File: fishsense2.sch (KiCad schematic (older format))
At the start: 15 parts, among them J1 Conn_02x10_Odd_Even, J10 USB_B_Micro, J5 USB3_A, J6 USB3_A, J7 USB3_A, J8 USB3_A, J9 Barrel_Jack, Q1 Q_NMOS_GSD, SW1 SW_Reed

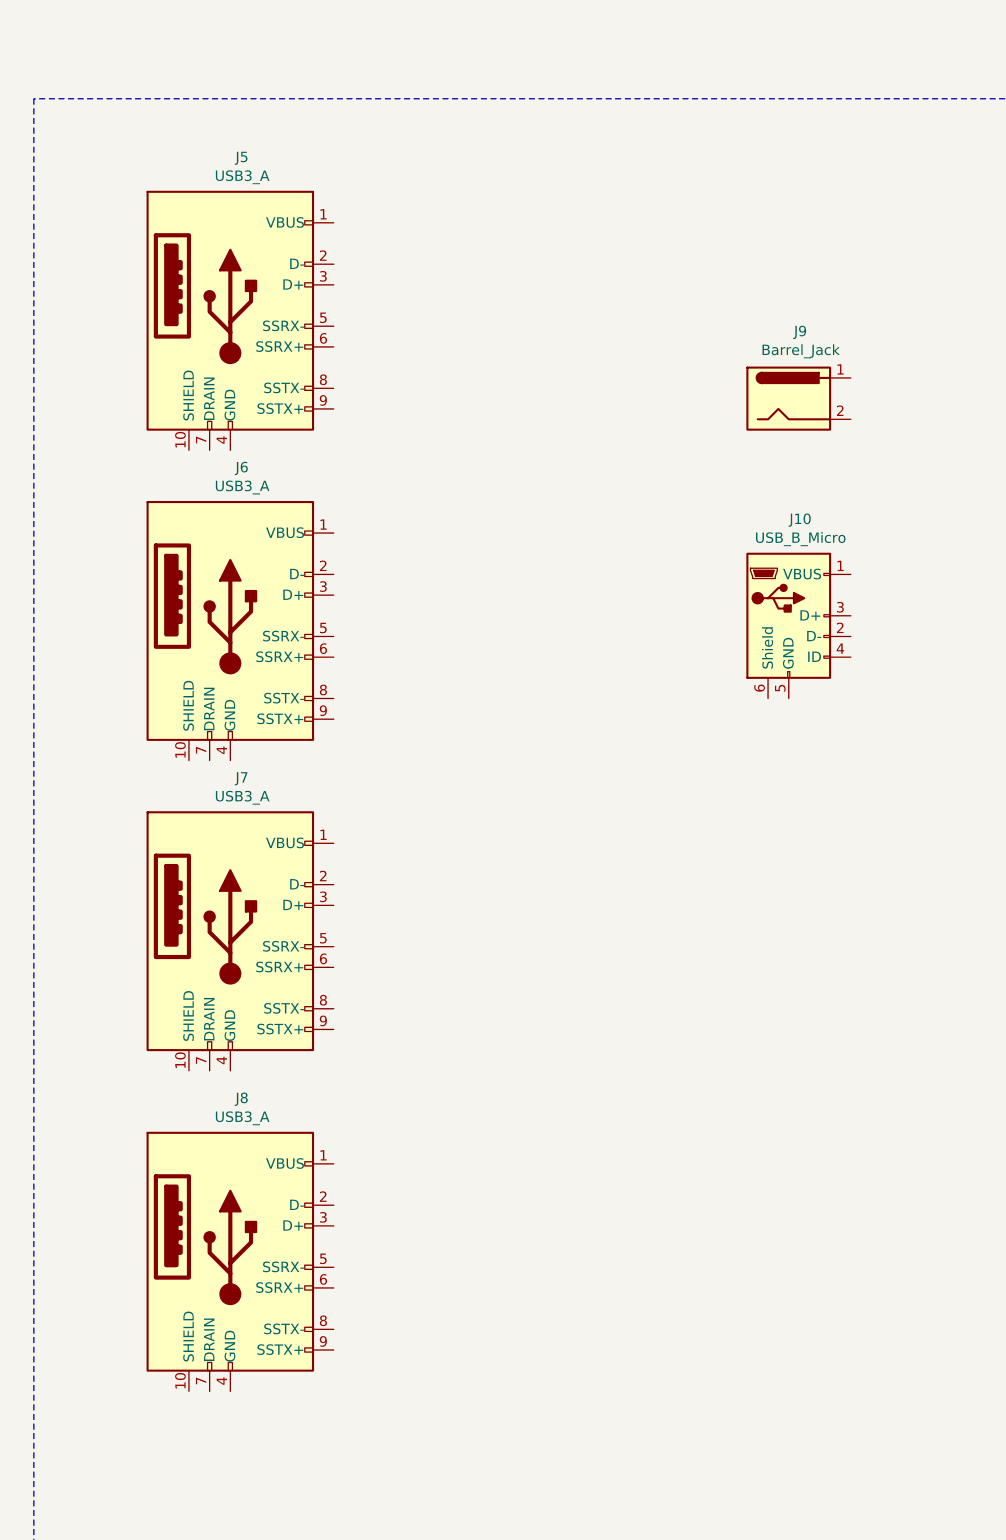
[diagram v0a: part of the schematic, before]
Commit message: Routed traces.
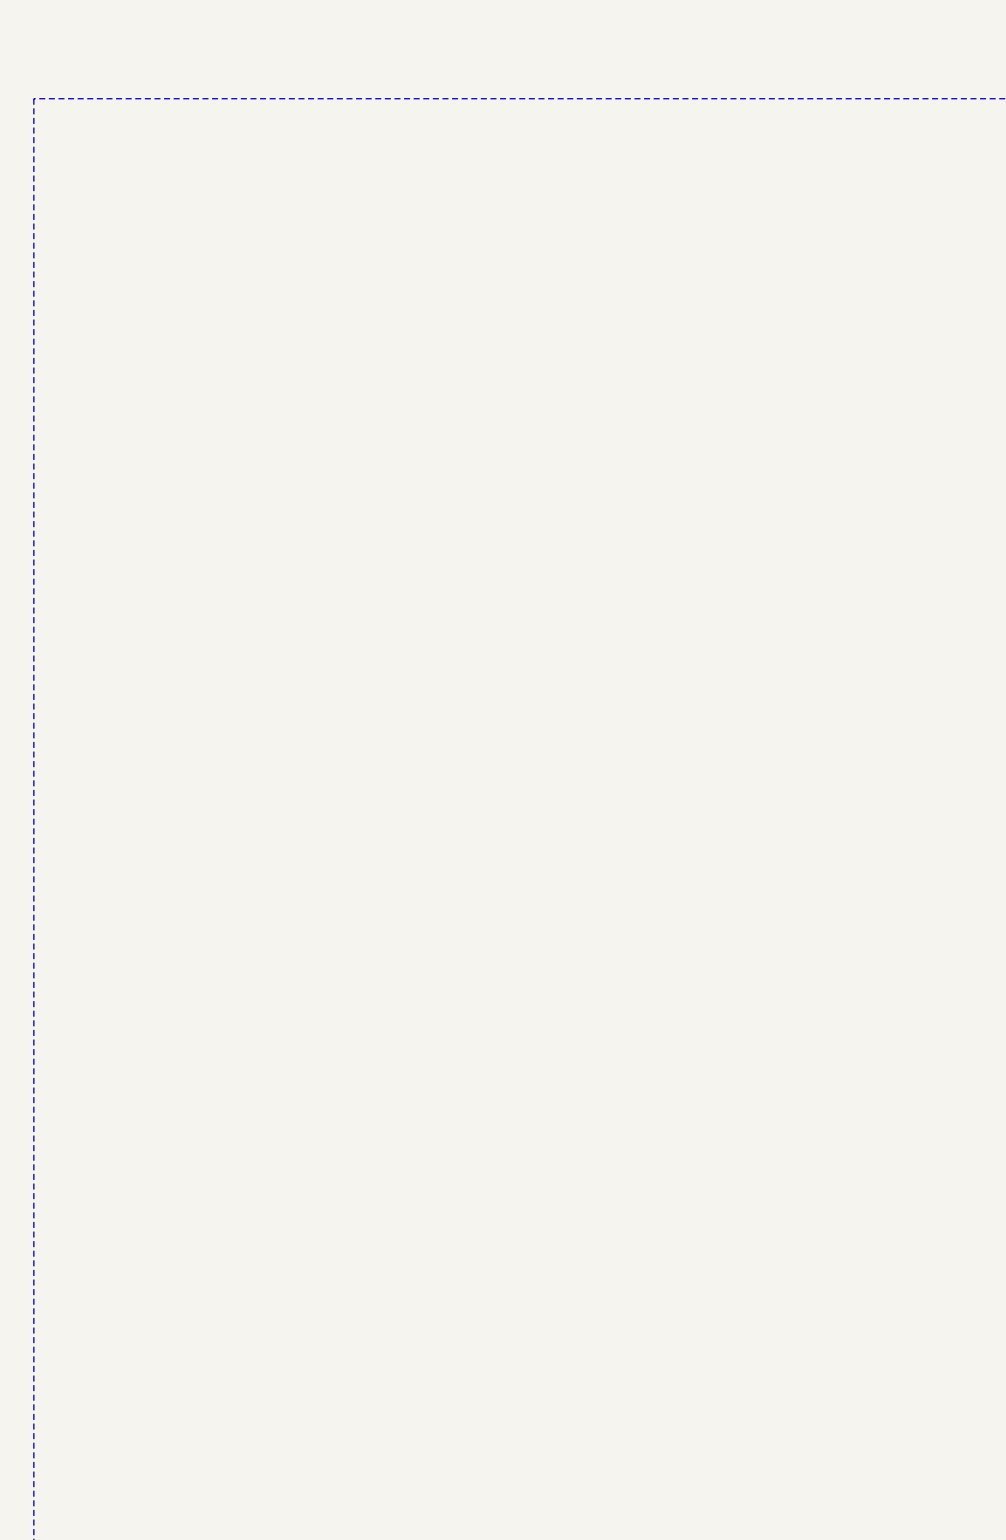
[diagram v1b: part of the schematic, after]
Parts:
- removed J10: USB_B_Micro, Connector_USB:USB_Micro-B_GCT_USB3076-30-A, symbol Connector:USB_B_Micro
- removed J5, J6, J7, J8: USB3_A, Connector_USB:USB3_A_Molex_48393-001, symbol Connector:USB3_A
- removed J9: Barrel_Jack, Connector_BarrelJack:BarrelJack_Horizontal, symbol Connector:Barrel_Jack
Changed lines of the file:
@@
 	11250 1900 4650 1900
-$Comp
-L Connector:USB3_A J5
-U 1 1 6196CE86
-P 5600 2900
-F 0 "J5" H 5657 3617 50  0000 C CNN
-F 1 "USB3_A" H 5657 3526 50  0000 C CNN
-F 2 "Connector_USB:USB3_A_Molex_48393-001" H 5750 3000 50  0001 C CNN
-F 3 "~" H 5750 3000 50  0001 C CNN
-	1    5600 2900
-	1    0    0    -1
-$EndComp
-$Comp
-L Connector:USB3_A J6
-U 1 1 6196EAC1
-P 5600 4400
-F 0 "J6" H 5657 5117 50  0000 C CNN
-F 1 "USB3_A" H 5657 5026 50  0000 C CNN
-F 2 "Connector_USB:USB3_A_Molex_48393-001" H 5750 4500 50  0001 C CNN
-F 3 "~" H 5750 4500 50  0001 C CNN
-	1    5600 4400
-	1    0    0    -1
-$EndComp
-$Comp
-L Connector:USB3_A J7
-U 1 1 619702D6
-P 5600 5900
-F 0 "J7" H 5657 6617 50  0000 C CNN
-F 1 "USB3_A" H 5657 6526 50  0000 C CNN
-F 2 "Connector_USB:USB3_A_Molex_48393-001" H 5750 6000 50  0001 C CNN
-F 3 "~" H 5750 6000 50  0001 C CNN
-	1    5600 5900
-	1    0    0    -1
-$EndComp
-$Comp
-L Connector:USB3_A J8
-U 1 1 619726A9
-P 5600 7450
-F 0 "J8" H 5657 8167 50  0000 C CNN
-F 1 "USB3_A" H 5657 8076 50  0000 C CNN
-F 2 "Connector_USB:USB3_A_Molex_48393-001" H 5750 7550 50  0001 C CNN
-F 3 "~" H 5750 7550 50  0001 C CNN
-	1    5600 7450
-	1    0    0    -1
-$EndComp
-$Comp
-L Connector:Barrel_Jack J9
-U 1 1 61974C09
-P 8300 3350
-F 0 "J9" H 8357 3675 50  0000 C CNN
-F 1 "Barrel_Jack" H 8357 3584 50  0000 C CNN
-F 2 "Connector_BarrelJack:BarrelJack_Horizontal" H 8350 3310 50  0001 C CNN
-F 3 "~" H 8350 3310 50  0001 C CNN
-	1    8300 3350
-	1    0    0    -1
-$EndComp
-$Comp
-L Connector:USB_B_Micro J10
-U 1 1 619775BF
-P 8300 4400
-F 0 "J10" H 8357 4867 50  0000 C CNN
-F 1 "USB_B_Micro" H 8357 4776 50  0000 C CNN
-F 2 "Connector_USB:USB_Micro-B_GCT_USB3076-30-A" H 8450 4350 50  0001 C CNN
-F 3 "~" H 8450 4350 50  0001 C CNN
-	1    8300 4400
-	1    0    0    -1
-$EndComp
 $Comp
 L Device:Q_NMOS_GSD Q1
